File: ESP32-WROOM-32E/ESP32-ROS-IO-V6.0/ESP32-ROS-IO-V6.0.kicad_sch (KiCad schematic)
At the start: 47 parts, among them J1 Conn_01x22_Socket, J16 XT60-M, J17 XT60-M, J2 Conn_01x22_Socket, J3 Conn_01x22_Socket, J4 Conn_01x22_Socket, J5 Conn_01x02_Pin, J6 Conn_01x02_Pin, SW1 SW1, SW2 SW2, SW3 SW3, SW4 SW4, SW5 SW5, SW6 SW6, SW7 SW7, SW8 SW8

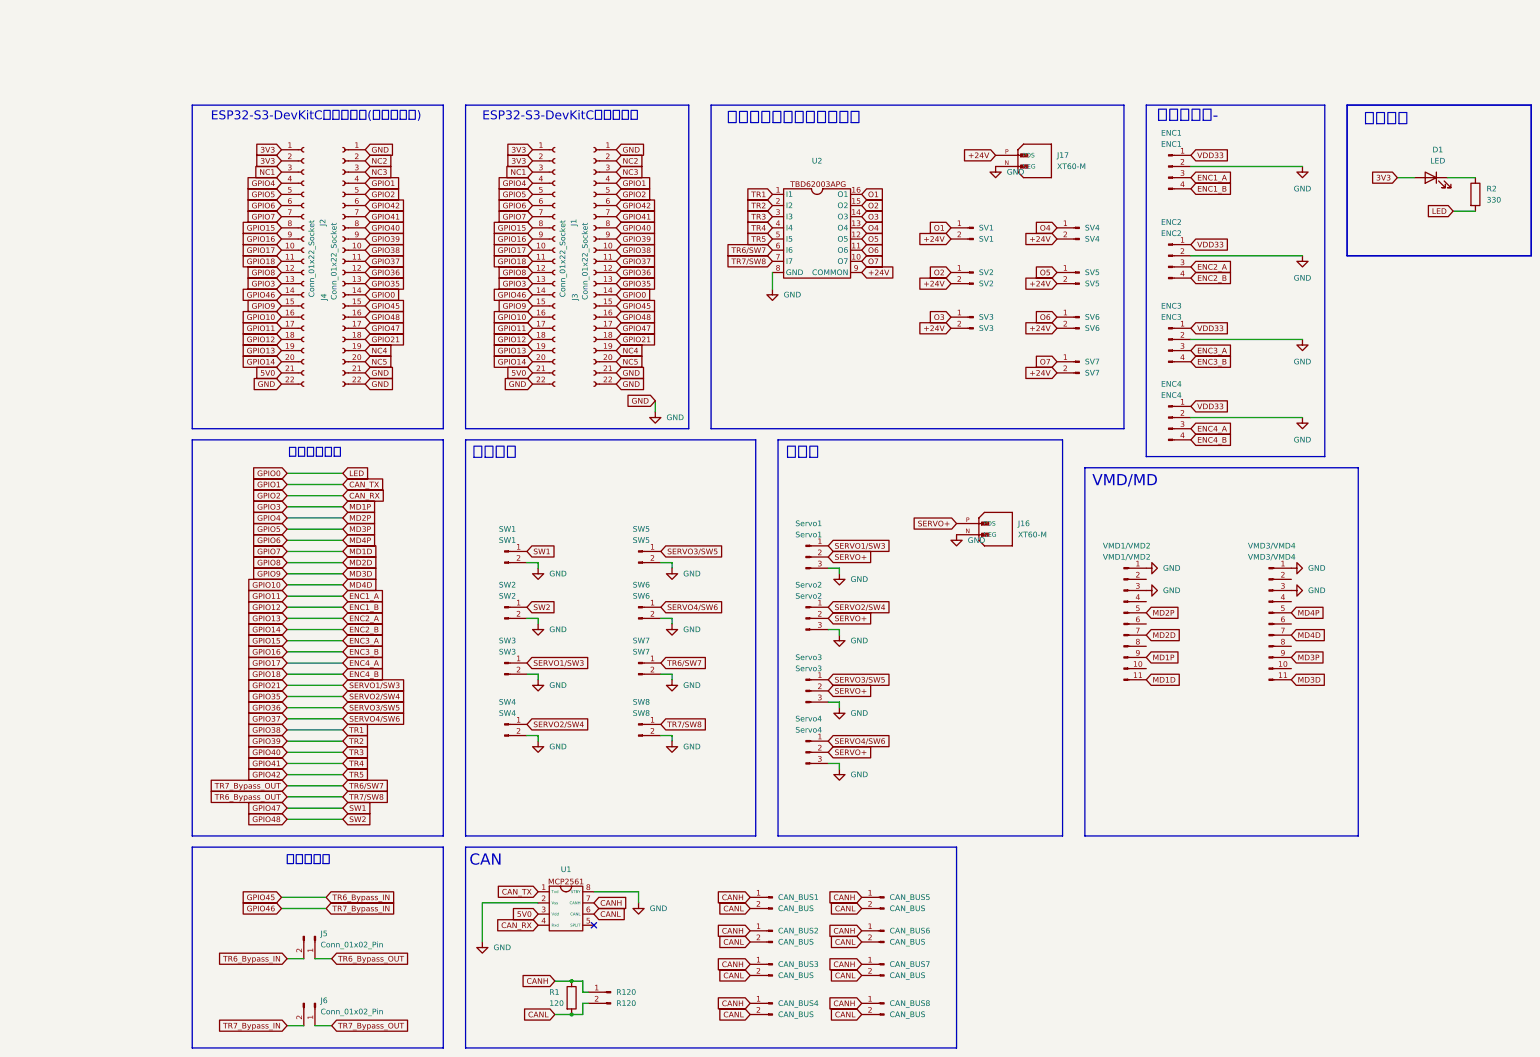
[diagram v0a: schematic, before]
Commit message: 回路図
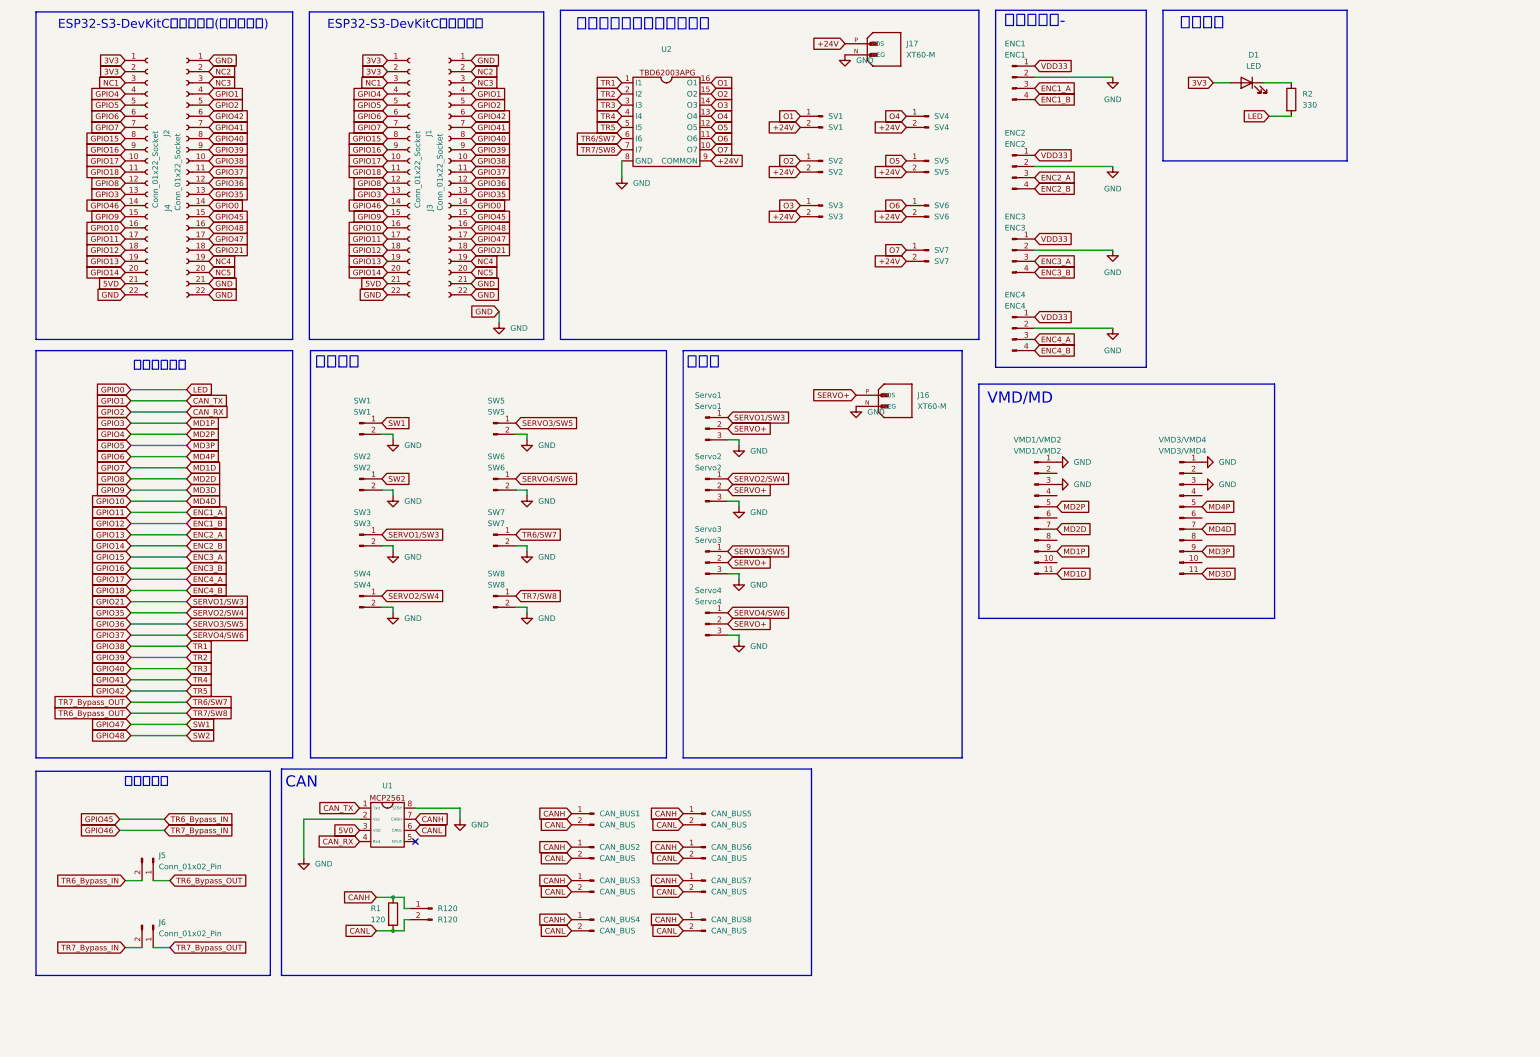
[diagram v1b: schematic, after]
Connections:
- net 5V0: no longer J1.21 (Pin_21), J2.21 (Pin_21)
- new net 5VD: J1.21 (Pin_21), J2.21 (Pin_21)
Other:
- moved on the sheet: J1, J2, J3, J4

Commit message: 回路図確定
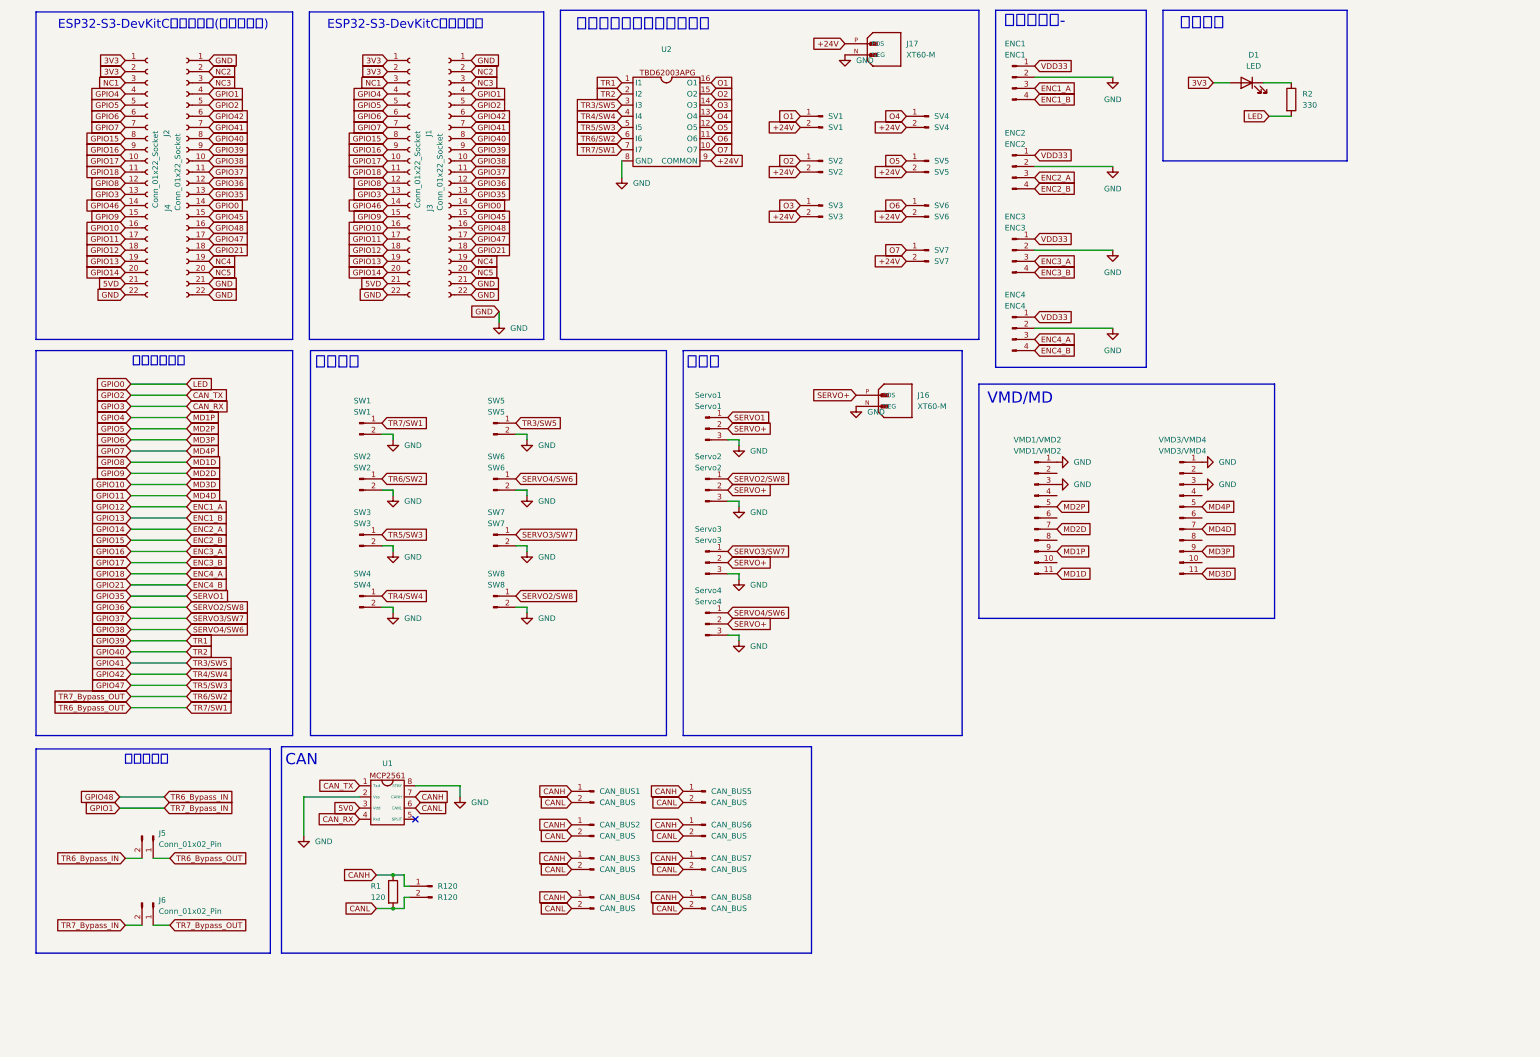
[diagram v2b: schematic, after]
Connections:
- net CAN_RX: now also J1.13 (Pin_13), J2.13 (Pin_13); no longer J3.5 (Pin_5), J4.5 (Pin_5)
- net CAN_TX: now also J3.5 (Pin_5), J4.5 (Pin_5); no longer J3.4 (Pin_4), J4.4 (Pin_4)
- net ENC1_A: now also J1.18 (Pin_18), J2.18 (Pin_18); no longer J1.17 (Pin_17), J2.17 (Pin_17)
- net ENC1_B: now also J1.19 (Pin_19), J2.19 (Pin_19); no longer J1.18 (Pin_18), J2.18 (Pin_18)
- net ENC2_A: now also J1.20 (Pin_20), J2.20 (Pin_20); no longer J1.19 (Pin_19), J2.19 (Pin_19)
- net ENC2_B: now also J1.8 (Pin_8), J2.8 (Pin_8); no longer J1.20 (Pin_20), J2.20 (Pin_20)
- net ENC3_A: now also J1.9 (Pin_9), J2.9 (Pin_9); no longer J1.8 (Pin_8), J2.8 (Pin_8)
- net ENC3_B: now also J1.10 (Pin_10), J2.10 (Pin_10); no longer J1.9 (Pin_9), J2.9 (Pin_9)
- net ENC4_A: now also J1.11 (Pin_11), J2.11 (Pin_11); no longer J1.10 (Pin_10), J2.10 (Pin_10)
- net ENC4_B: now also J3.18 (Pin_18), J4.18 (Pin_18); no longer J1.11 (Pin_11), J2.11 (Pin_11)
- net GPIO10: now also VMD3/VMD4.11 (Pin_11); no longer VMD3/VMD4.7 (Pin_7)
- net GPIO35: now also Servo1.1 (Pin_1); no longer SW4.1 (Pin_1), Servo2.1 (Pin_1)
- net GPIO36: now also SW8.1 (Pin_1), Servo2.1 (Pin_1); no longer SW5.1 (Pin_1), Servo3.1 (Pin_1)
- net GPIO37: now also SW7.1 (Pin_1), Servo3.1 (Pin_1); no longer SW6.1 (Pin_1), Servo4.1 (Pin_1)
- net GPIO38: now also SW6.1 (Pin_1), Servo4.1 (Pin_1); no longer U2.1 (I1)
- net GPIO39: now also U2.1 (I1); no longer U2.2 (I2)
- net GPIO4: now also VMD1/VMD2.9 (Pin_9); no longer VMD1/VMD2.5 (Pin_5)
- net GPIO40: now also U2.2 (I2); no longer U2.3 (I3)
- net GPIO41: now also SW5.1 (Pin_1), U2.3 (I3); no longer U2.4 (I4)
- net GPIO42: now also SW4.1 (Pin_1), U2.4 (I4); no longer U2.5 (I5)
- net GPIO45: no longer J5.2 (Pin_2)
- net GPIO46: no longer J6.2 (Pin_2)
- net GPIO47: now also SW3.1 (Pin_1), U2.5 (I5); no longer SW1.1 (Pin_1)
- net GPIO48: now also J5.2 (Pin_2); no longer SW2.1 (Pin_1)
- net GPIO5: now also VMD1/VMD2.5 (Pin_5); no longer VMD3/VMD4.9 (Pin_9)
- net GPIO6: now also VMD3/VMD4.9 (Pin_9); no longer VMD3/VMD4.5 (Pin_5)
- net GPIO7: now also VMD3/VMD4.5 (Pin_5); no longer VMD1/VMD2.11 (Pin_11)
- net GPIO8: now also VMD1/VMD2.11 (Pin_11); no longer VMD1/VMD2.7 (Pin_7)
- net GPIO9: now also VMD1/VMD2.7 (Pin_7); no longer VMD3/VMD4.11 (Pin_11)
- net TR6_Bypass_OUT: now also SW1.1 (Pin_1); no longer SW8.1 (Pin_1)
- removed net GPIO21: J3.18 (Pin_18), J4.18 (Pin_18), SW3.1 (Pin_1), Servo1.1 (Pin_1)
- removed net GPIO3: J1.13 (Pin_13), J2.13 (Pin_13), VMD1/VMD2.9 (Pin_9)
- net TR6/SW7 renamed TR6/SW2
- net TR6/SW2: now also SW2.1 (Pin_1); no longer SW7.1 (Pin_1)
- new net GPIO1: J3.4 (Pin_4), J4.4 (Pin_4), J6.2 (Pin_2)
- new net GPIO11: J1.17 (Pin_17), J2.17 (Pin_17), VMD3/VMD4.7 (Pin_7)
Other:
- moved on the sheet: CAN_BUS1, CAN_BUS2, CAN_BUS3, CAN_BUS4, CAN_BUS5, CAN_BUS6, CAN_BUS7, CAN_BUS8, J5, J6, R1, R120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

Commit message: フットプリント割り当て
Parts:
- J1, J2, J3, J4: footprint (none) -> Connector_PinSocket_2.54mm:PinSocket_1x19_P2.54mm_Vertical
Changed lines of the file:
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@@
 			)
 		)
-		(property "Footprint" ""
+		(property "Footprint" "Connector_PinSocket_2.54mm:PinSocket_1x19_P2.54mm_Vertical"
 			(at 100.33 52.07 0)
 			(effects
@@
 			)
 		)
-		(property "Footprint" ""
+		(property "Footprint" "Connector_PinSocket_2.54mm:PinSocket_1x19_P2.54mm_Vertical"
 			(at 49.53 52.07 0)
 			(effects
@@
 			)
 		)
-		(property "Footprint" ""
+		(property "Footprint" "Connector_PinSocket_2.54mm:PinSocket_1x19_P2.54mm_Vertical"
 			(at 40.64 52.07 0)
 			(effects
@@
 			)
 		)
-		(property "Footprint" ""
+		(property "Footprint" "Connector_PinSocket_2.54mm:PinSocket_1x19_P2.54mm_Vertical"
 			(at 109.22 52.07 0)
 			(effects
